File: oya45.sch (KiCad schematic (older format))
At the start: 94 parts, among them U1 Elite-C

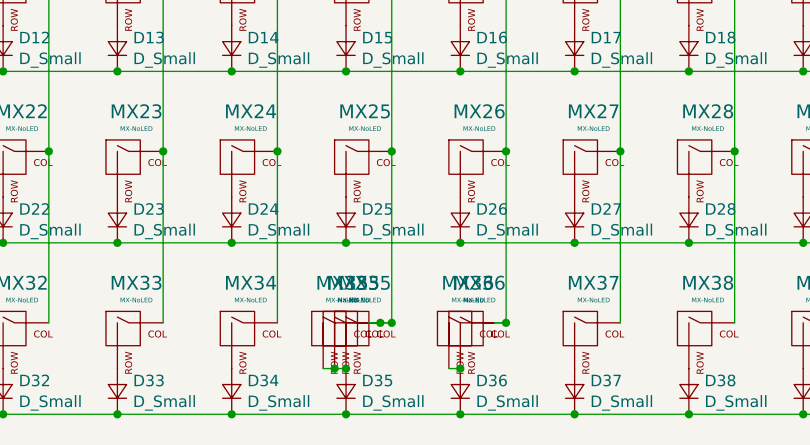
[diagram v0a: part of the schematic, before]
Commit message: Schematics finished final
fixed duplicates
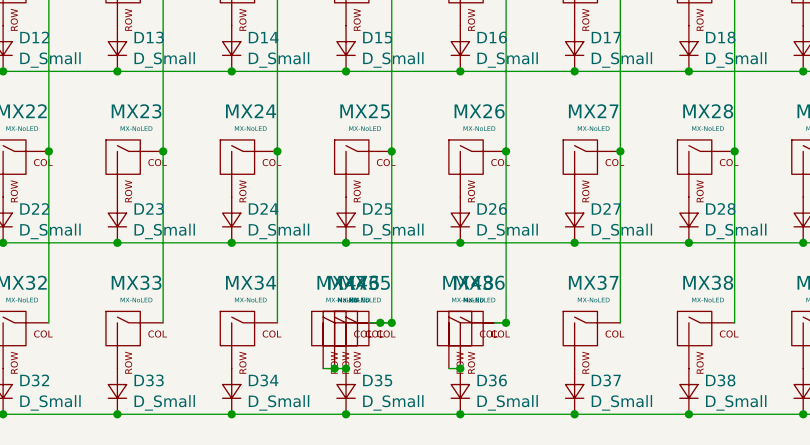
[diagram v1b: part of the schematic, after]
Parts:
- renumbered MX35 to MX46, MX35 to MX47, MX36 to MX48
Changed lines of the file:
@@
 $EndComp
 $Comp
-L MX_Alps_Hybrid:MX-NoLED MX36
+L MX_Alps_Hybrid:MX-NoLED MX48
 U 1 1 61374F37
 P 8050 4850
-F 0 "MX36" H 8083 5073 60  0000 C CNN
+F 0 "MX48" H 8083 5073 60  0000 C CNN
 F 1 "MX-NoLED" H 8083 4999 20  0000 C CNN
 F 2 "" H 7425 4825 60  0001 C CNN
@@
 $EndComp
 $Comp
-L MX_Alps_Hybrid:MX-NoLED MX35
+L MX_Alps_Hybrid:MX-NoLED MX46
 U 1 1 61375469
 P 7550 4850
-F 0 "MX35" H 7583 5073 60  0000 C CNN
+F 0 "MX46" H 7583 5073 60  0000 C CNN
 F 1 "MX-NoLED" H 7583 4999 20  0000 C CNN
 F 2 "" H 6925 4825 60  0001 C CNN
@@
 $EndComp
 $Comp
-L MX_Alps_Hybrid:MX-NoLED MX35
+L MX_Alps_Hybrid:MX-NoLED MX47
 U 1 1 61377FE9
 P 7500 4850
-F 0 "MX35" H 7533 5073 60  0000 C CNN
+F 0 "MX47" H 7533 5073 60  0000 C CNN
 F 1 "MX-NoLED" H 7533 4999 20  0000 C CNN
 F 2 "" H 6875 4825 60  0001 C CNN
